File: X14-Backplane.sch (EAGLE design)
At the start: 27 parts, among them J2 PXC-PTSM-04-RA-1778641, J3 PXC-8-RA-1778683, J8 PXC-8-RA-1778683

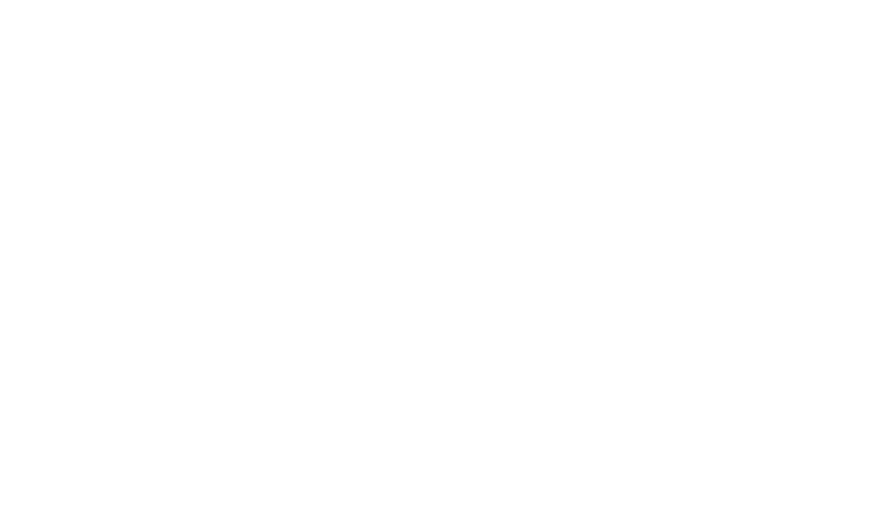
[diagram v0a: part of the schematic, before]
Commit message: afawevvew
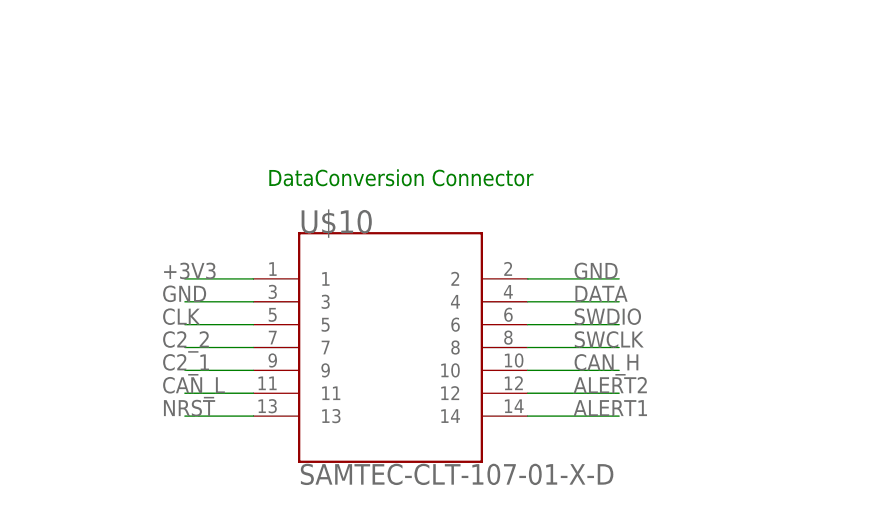
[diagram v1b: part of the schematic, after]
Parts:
- added U$10: BACKPLANE->DATACONV, CONN, DataConversion-Backplane Connector- SAMTEC CLT-107-01-F-D:BACKPLANE->DATACONV
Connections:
- new net +3V3: U$10.1
- new net ALERT1: U$10.14
- new net ALERT2: U$10.12
- new net GND: U$10.2, U$10.3
- new net SWCLK: U$10.8
- new net SWDIO: U$10.6
- net C2_1: now also U$10.9
- net C2_2: now also U$10.7
- net CAN_H: now also U$10.10
- net CAN_L: now also U$10.11
- net CLK: now also U$10.5
- net DATA: now also U$10.4
- net NRST: now also U$10.13
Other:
- note added: "DataConversion Connector"
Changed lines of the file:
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@@
 <?xml version="1.0" encoding="utf-8"?>
 <!DOCTYPE eagle SYSTEM "eagle.dtd">
-<eagle version="9.5.0">
+<eagle version="9.6.2">
 <drawing>
 <settings>
@@
 <part name="J8" library="Phoenix Contact PTSM 8 pin" deviceset="PXC-8-RA-1778683" device="" package3d_urn="urn:adsk.eagle:package:25224885/2"/>
 <part name="U$9" library="PI-SHIELD, Solenoid-Backplane" deviceset="7X_CONN" device=""/>
+<part name="U$10" library="CONN, DataConversion-Backplane Connector- SAMTEC CLT-107-01-F-D" deviceset="BACKPLANE-&gt;DATACONV" device=""/>
 </parts>
 <sheets>
@@
 <text x="72.67" y="-23.96" size="1.778" layer="91">PI Shield Connector</text>
 <text x="191.02" y="-19.88" size="1.778" layer="91">CAN io</text>
+<text x="34.57" y="-73.49" size="1.778" layer="91">DataConversion Connector</text>
 </plain>
 <instances>
@@
 </instance>
 <instance part="U$9" gate="G$1" x="83.82" y="-39.37" smashed="yes"/>
+<instance part="U$10" gate="G$1" x="38.1" y="-83.82" smashed="yes">
+<attribute name="NAME" x="38.1" y="-78.74" size="2.54" layer="95"/>
+</instance>
 </instances>
 <busses>
@@
 <label x="67.31" y="-48.26" size="1.778" layer="95"/>
 </segment>
+<segment>
+<wire x1="73.66" y1="-93.98" x2="63.5" y2="-93.98" width="0.1524" layer="91"/>
+<label x="68.58" y="-93.98" size="1.778" layer="95"/>
+<pinref part="U$10" gate="G$1" pin="10"/>
+</segment>
 </net>
 <net name="CAN_L" class="0">
@@
 <wire x1="91.44" y1="-48.26" x2="100.33" y2="-48.26" width="0.1524" layer="91"/>
 <label x="92.71" y="-48.26" size="1.778" layer="95"/>
+</segment>
+<segment>
+<wire x1="25.4" y1="-96.52" x2="33.02" y2="-96.52" width="0.1524" layer="91"/>
+<label x="22.86" y="-96.52" size="1.778" layer="95"/>
+<pinref part="U$10" gate="G$1" pin="11"/>
 </segment>
 </net>
@@
 <junction x="243.84" y="60.96"/>
 </segment>
+<segment>
+<wire x1="33.02" y1="-99.06" x2="25.4" y2="-99.06" width="0.1524" layer="91"/>
+<label x="22.86" y="-99.06" size="1.778" layer="95"/>
+<pinref part="U$10" gate="G$1" pin="13"/>
+</segment>
 </net>
 <net name="ESCID_1" class="0">
@@
 <label x="105" y="34.4" size="1.778" layer="95"/>
 </segment>
+<segment>
+<wire x1="33.02" y1="-88.9" x2="25.4" y2="-88.9" width="0.1524" layer="91"/>
+<label x="22.86" y="-88.9" size="1.778" layer="95"/>
+<pinref part="U$10" gate="G$1" pin="5"/>
+</segment>
 </net>
 <net name="C2_1" class="0">
@@
 <label x="104.1" y="31.8" size="1.778" layer="95"/>
 </segment>
+<segment>
+<wire x1="33.02" y1="-93.98" x2="25.4" y2="-93.98" width="0.1524" layer="91"/>
+<label x="22.86" y="-93.98" size="1.778" layer="95"/>
+<pinref part="U$10" gate="G$1" pin="9"/>
+</segment>
 </net>
 <net name="C2_2" class="0">
@@
 <label x="104.3" y="29.3" size="1.778" layer="95"/>
 </segment>
+<segment>
+<wire x1="25.4" y1="-91.44" x2="33.02" y2="-91.44" width="0.1524" layer="91"/>
+<label x="22.86" y="-91.44" size="1.778" layer="95"/>
+<pinref part="U$10" gate="G$1" pin="7"/>
+</segment>
 </net>
 <net name="DATA" class="0">
@@
 <wire x1="95.98" y1="41.78" x2="109.81" y2="41.78" width="0.1524" layer="91"/>
 <label x="103.2" y="42.1" size="1.778" layer="95"/>
+</segment>
+<segment>
+<wire x1="63.5" y1="-86.36" x2="73.66" y2="-86.36" width="0.1524" layer="91"/>
+<label x="68.58" y="-86.36" size="1.778" layer="95"/>
+<pinref part="U$10" gate="G$1" pin="4"/>
 </segment>
 </net>
@@
 </segment>
 </net>
+<net name="GND" class="0">
+<segment>
+<wire x1="33.02" y1="-86.36" x2="25.4" y2="-86.36" width="0.1524" layer="91"/>
+<label x="22.86" y="-86.36" size="1.778" layer="95"/>
+<pinref part="U$10" gate="G$1" pin="3"/>
+</segment>
+<segment>
+<wire x1="63.5" y1="-83.82" x2="73.66" y2="-83.82" width="0.1524" layer="91"/>
+<label x="68.58" y="-83.82" size="1.778" layer="95"/>
+<pinref part="U$10" gate="G$1" pin="2"/>
+</segment>
+</net>
+<net name="+3V3" class="0">
+<segment>
+<wire x1="33.02" y1="-83.82" x2="25.4" y2="-83.82" width="0.1524" layer="91"/>
+<label x="22.86" y="-83.82" size="1.778" layer="95"/>
+<pinref part="U$10" gate="G$1" pin="1"/>
+</segment>
+</net>
+<net name="SWDIO" class="0">
+<segment>
+<wire x1="63.5" y1="-88.9" x2="73.66" y2="-88.9" width="0.1524" layer="91"/>
+<label x="68.58" y="-88.9" size="1.778" layer="95"/>
+<pinref part="U$10" gate="G$1" pin="6"/>
+</segment>
+</net>
+<net name="SWCLK" class="0">
+<segment>
+<wire x1="63.5" y1="-91.44" x2="73.66" y2="-91.44" width="0.1524" layer="91"/>
+<label x="68.58" y="-91.44" size="1.778" layer="95"/>
+<pinref part="U$10" gate="G$1" pin="8"/>
+</segment>
+</net>
+<net name="ALERT2" class="0">
+<segment>
+<wire x1="73.66" y1="-96.52" x2="63.5" y2="-96.52" width="0.1524" layer="91"/>
+<label x="68.58" y="-96.52" size="1.778" layer="95"/>
+<pinref part="U$10" gate="G$1" pin="12"/>
+</segment>
+</net>
+<net name="ALERT1" class="0">
+<segment>
+<wire x1="63.5" y1="-99.06" x2="73.66" y2="-99.06" width="0.1524" layer="91"/>
+<label x="68.58" y="-99.06" size="1.778" layer="95"/>
+<pinref part="U$10" gate="G$1" pin="14"/>
+</segment>
+</net>
